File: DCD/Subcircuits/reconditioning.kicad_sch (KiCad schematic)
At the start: 36 parts, among them IC1 830S21AMI-01LF, IC2 830S21AMI-01LF, U15 MC100EP31DTG, U16 MC100EP31DTG, U7 LP2985-33DBVR, U8 CDCLVC1104PWR, Y1 SiT8208AI-21-33E-50.000000

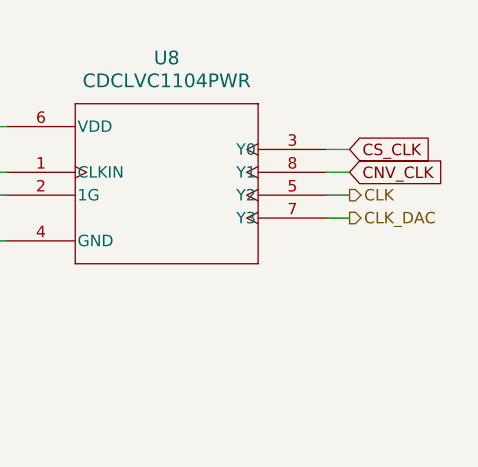
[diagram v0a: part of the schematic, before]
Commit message: Layout mostly done
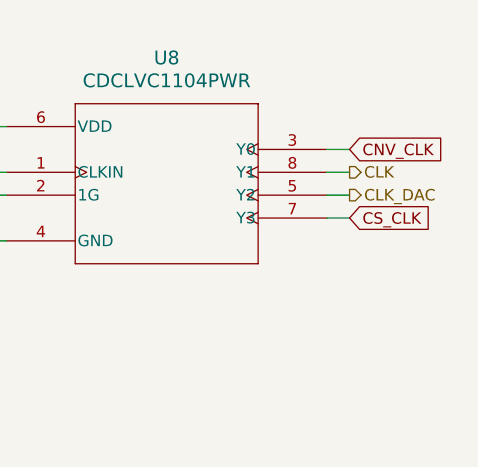
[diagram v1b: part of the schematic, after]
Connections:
- net CLK: now also U8.8 (Y1); no longer U8.5 (Y2)
- net CLK_DAC: now also U8.5 (Y2); no longer U8.7 (Y3)
- net CNV_CLK: now also U8.3 (Y0); no longer U8.8 (Y1)
- net CS_CLK: now also U8.7 (Y3); no longer U8.3 (Y0)
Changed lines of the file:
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@@
+		)
+	)
+	(global_label "3V3_CLK"
+		(shape input)
+		(at 80.01 29.21 90)
+		(fields_autoplaced yes)
+		(effects
+			(font
+				(size 1.27 1.27)
+			)
+			(justify left)
+		)
+		(property "Intersheetrefs" "${INTERSHEET_REFS}"
+			(at 80.01 18.1815 90)
+			(effects
+				(font
+					(size 1.27 1.27)
+				)
+				(justify left)
+				(hide yes)
+			)
+		)
+	)
+	(global_label "3V3_CLK"
+		(shape input)
+		(at 194.31 125.73 90)
+		(fields_autoplaced yes)
+		(effects
+			(font
+				(size 1.27 1.27)
+			)
+			(justify left)
+		)
+		(property "Intersheetrefs" "${INTERSHEET_REFS}"
+			(at 194.31 114.7015 90)
+			(effects
+				(font
+					(size 1.27 1.27)
+				)
+				(justify left)
+				(hide yes)
+			)
+		)
+	)
+	(global_label "CS_CLK"
+		(shape input)
+		(at 256.54 39.37 0)
+		(fields_autoplaced yes)
+		(effects
+			(font
+				(size 1.27 1.27)
+			)
+			(justify left)
+		)
+		(property "Intersheetrefs" "${INTERSHEET_REFS}"
+			(at 266.5404 39.37 0)
+			(effects
+				(font
+					(size 1.27 1.27)
+				)
+				(justify left)
+				(hide yes)
+			)
+		)
+	)
+	(global_label "3V3_CLK"
+		(shape input)
+		(at 30.48 125.73 90)
+		(fields_autoplaced yes)
+		(effects
+			(font
+				(size 1.27 1.27)
+			)
+			(justify left)
+		)
+		(property "Intersheetrefs" "${INTERSHEET_REFS}"
+			(at 30.48 114.7015 90)
+			(effects
+				(font
+					(size 1.27 1.27)
+				)
+				(justify left)
+				(hide yes)
+			)
 		)
 	)
 	(global_label "CNV_CLK"
 		(shape input)
+		(at 256.54 31.75 0)
+		(fields_autoplaced yes)
+		(effects
+			(font
+				(size 1.27 1.27)
+			)
+			(justify left)
+		)
+		(property "Intersheetrefs" "${INTERSHEET_REFS}"
+			(at 267.75 31.75 0)
+			(effects
+				(font
+					(size 1.27 1.27)
+				)
+				(justify left)
+				(hide yes)
+			)
+		)
+	)
+	(global_label "CNV_CLK"
+		(shape input)
+		(at 71.12 146.05 180)
+		(fields_autoplaced yes)
+		(effects
+			(font
+				(size 1.27 1.27)
+			)
+			(justify right)
+		)
+		(property "Intersheetrefs" "${INTERSHEET_REFS}"
+			(at 59.91 146.05 0)
+			(effects
+				(font
+					(size 1.27 1.27)
+				)
+				(justify right)
+				(hide yes)
+			)
+		)
+	)
+	(hierarchical_label "CLK"
+		(shape output)
 		(at 256.54 34.29 0)
-		(fields_autoplaced yes)
-		(effects
-			(font
-				(size 1.27 1.27)
-			)
-			(justify left)
-		)
-		(property "Intersheetrefs" "${INTERSHEET_REFS}"
-			(at 267.75 34.29 0)
-			(effects
-				(font
-					(size 1.27 1.27)
-				)
-				(justify left)
-				(hide yes)
-			)
-		)
-	)
-	(global_label "3V3_CLK"
-		(shape input)
-		(at 80.01 29.21 90)
-		(fields_autoplaced yes)
-		(effects
-			(font
-				(size 1.27 1.27)
-			)
-			(justify left)
-		)
-		(property "Intersheetrefs" "${INTERSHEET_REFS}"
-			(at 80.01 18.1815 90)
-			(effects
-				(font
-					(size 1.27 1.27)
-				)
-				(justify left)
-				(hide yes)
-			)
-		)
-	)
-	(global_label "3V3_CLK"
-		(shape input)
-		(at 194.31 125.73 90)
-		(fields_autoplaced yes)
-		(effects
-			(font
-				(size 1.27 1.27)
-			)
-			(justify left)
-		)
-		(property "Intersheetrefs" "${INTERSHEET_REFS}"
-			(at 194.31 114.7015 90)
-			(effects
-				(font
-					(size 1.27 1.27)
-				)
-				(justify left)
-				(hide yes)
-			)
-		)
-	)
-	(global_label "CS_CLK"
-		(shape input)
-		(at 256.54 31.75 0)
-		(fields_autoplaced yes)
-		(effects
-			(font
-				(size 1.27 1.27)
-			)
-			(justify left)
-		)
-		(property "Intersheetrefs" "${INTERSHEET_REFS}"
-			(at 266.5404 31.75 0)
-			(effects
-				(font
-					(size 1.27 1.27)
-				)
-				(justify left)
-				(hide yes)
-			)
-		)
-	)
-	(global_label "3V3_CLK"
-		(shape input)
-		(at 30.48 125.73 90)
-		(fields_autoplaced yes)
-		(effects
-			(font
-				(size 1.27 1.27)
-			)
-			(justify left)
-		)
-		(property "Intersheetrefs" "${INTERSHEET_REFS}"
-			(at 30.48 114.7015 90)
-			(effects
-				(font
-					(size 1.27 1.27)
-				)
-				(justify left)
-				(hide yes)
-			)
-		)
-	)
-	(global_label "CNV_CLK"
-		(shape input)
-		(at 71.12 146.05 180)
-		(fields_autoplaced yes)
-		(effects
-			(font
-				(size 1.27 1.27)
-			)
-			(justify right)
-		)
-		(property "Intersheetrefs" "${INTERSHEET_REFS}"
-			(at 59.91 146.05 0)
-			(effects
-				(font
-					(size 1.27 1.27)
-				)
-				(justify right)
-				(hide yes)
-			)
+		(effects
+			(font
+				(size 1.27 1.27)
+			)
+			(justify left)
 		)
 	)
@@
 		)
 	)
+	(hierarchical_label "CLK_DAC"
+		(shape output)
+		(at 256.54 36.83 0)
+		(effects
+			(font
+				(size 1.27 1.27)
+			)
+			(justify left)
+		)
+	)
 	(hierarchical_label "DGND"
 		(shape input)
@@
 		)
 	)
-	(hierarchical_label "CLK_DAC"
-		(shape output)
-		(at 256.54 39.37 0)
-		(effects
-			(font
-				(size 1.27 1.27)
-			)
-			(justify left)
-		)
-	)
 	(hierarchical_label "7V"
 		(shape input)
@@
 		(effects
 			(font
-				(size 1.27 1.27)
-			)
-			(justify left)
-		)
-	)
-	(hierarchical_label "CLK"
-		(shape output)
-		(at 256.54 36.83 0)
-		(effects
-			(font
